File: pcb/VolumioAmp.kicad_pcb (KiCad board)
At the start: 2 copper layers, 172.1 x 71.1 mm, 121 parts, among them IC1 PCM2706, IC2 WM8804GEDS_V, J1 L829-1J1T-43, J2 USB4500-03-0-A_REVA, J3 24v Input, J4 Screw_Terminal_01x04, J5 Conn_Coaxial, Q1 DMP3013SFV-7, U1 74LVC1G07SE-7, U2 TPD4EUSB30, U3 TPD4EUSB30, U4 FSUSB42MUX, U5 24AA02-OT, U6 AP64501SP-13, U7 LT1761-3.3, U8 MA12040PXUMA1, Y1 12Mhz, Y2 12Mhz

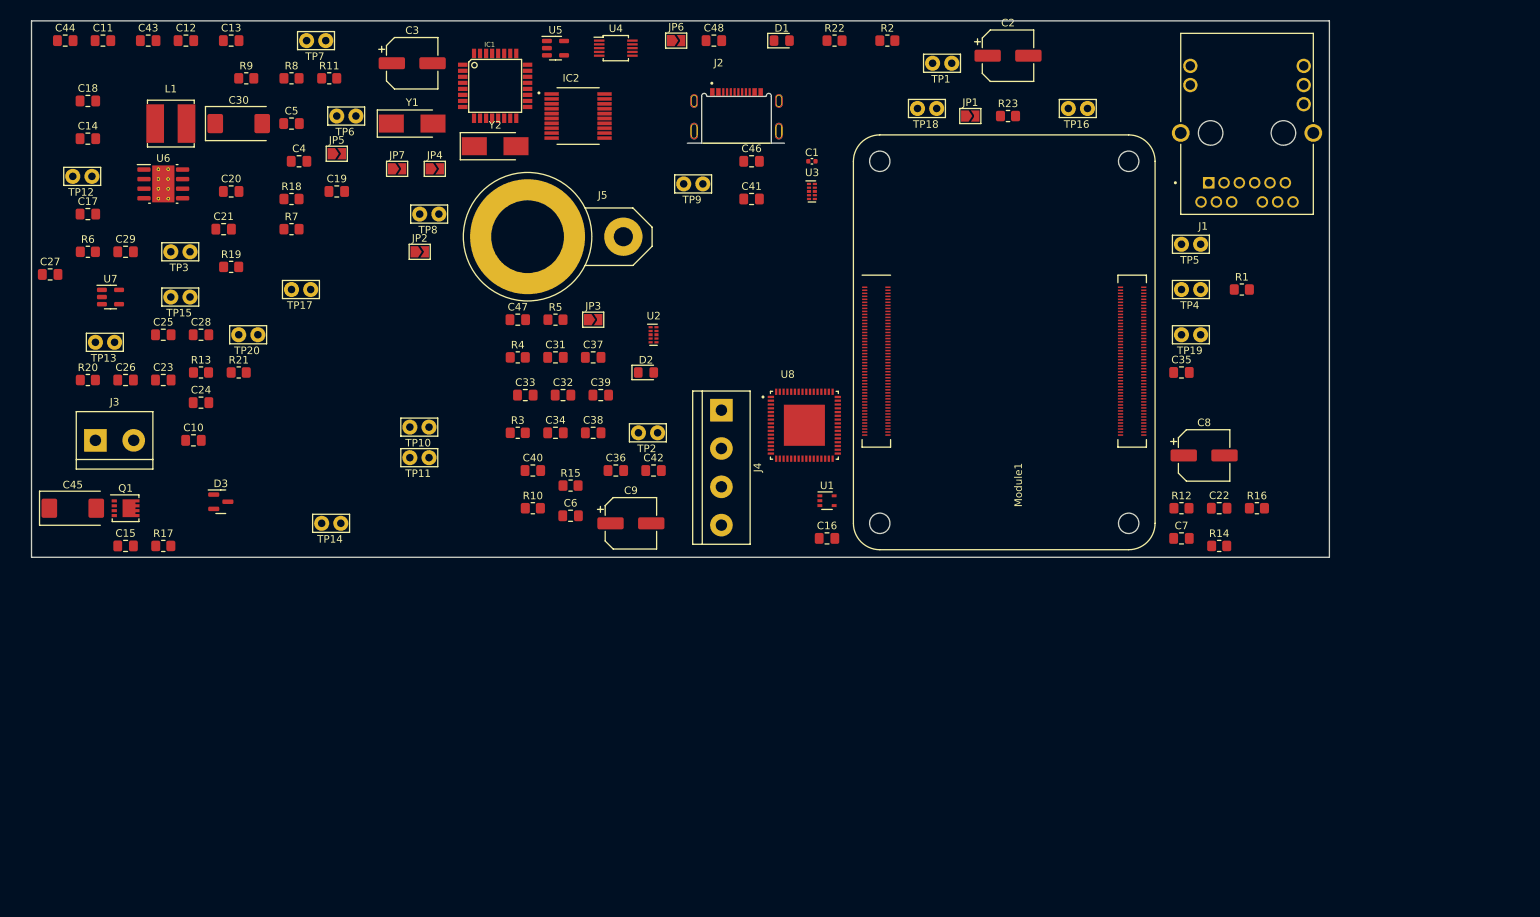
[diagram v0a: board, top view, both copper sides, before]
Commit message: - placing components
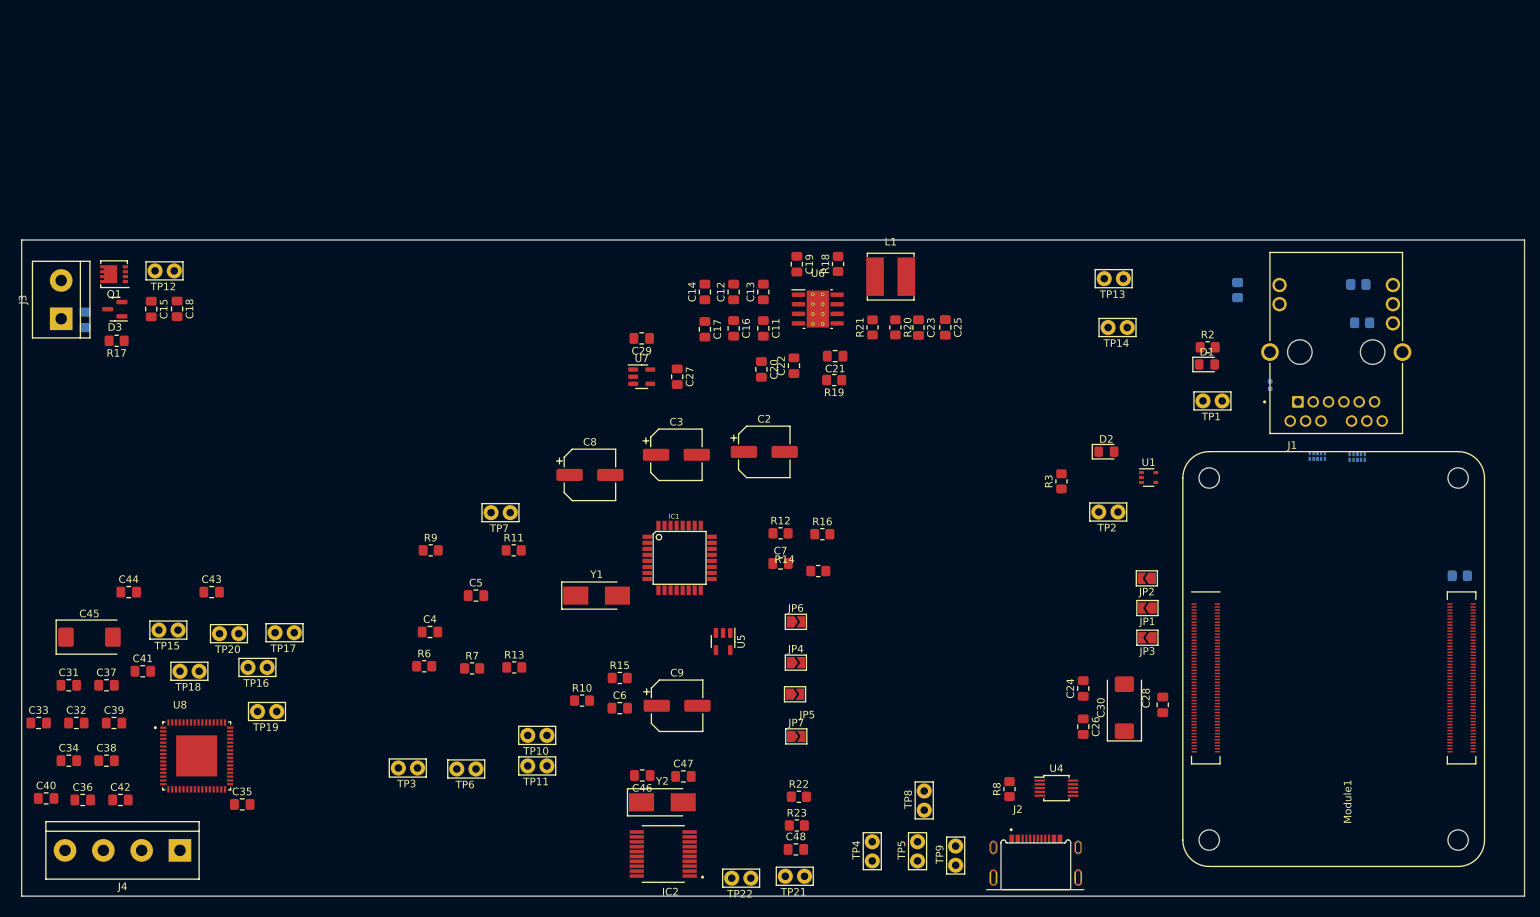
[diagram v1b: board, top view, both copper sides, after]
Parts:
- removed J5: Conn_Coaxial, Connector_Coaxial:BNC_PanelMountable_Vertical
- added R24: 470R, Resistor_SMD:R_0805_2012Metric_Pad1.20x1.40mm_HandSolder, B.Cu at (209.5, 59.3)
- added TP21: TestPoint, TestPoint:TestPoint_Bridge_Pitch2.54mm_Drill1.0mm, F.Cu at (133.5, 137.8)
- added TP22: TestPoint, TestPoint:TestPoint_Bridge_Pitch2.54mm_Drill1.0mm, F.Cu at (126.4, 138.0)
- C1, C10, R1, R4, R5, U2, U3: moved to B.Cu
- R8: value 2.2K 1% -> 2.2K
- moved C30 140.7 mm to (178.4, 115.4), turned to 90 degrees
- moved C35 137.1 mm to (61.5, 128.3)
- moved C28 136.6 mm to (183.5, 115.1), turned to 90 degrees
- moved C26 135.0 mm to (173.0, 118.0), turned to -90 degrees
- moved TP13 134.0 mm to (175.8, 58.6)
- moved R8 134.0 mm to (163.2, 126.2), turned to 90 degrees
- moved TP19 132.3 mm to (63.5, 116.0)
- moved TP16 131.6 mm to (62.2, 110.1)
- moved TP18 123.0 mm to (53.2, 110.6)
- moved C24 123.0 mm to (173.0, 112.9), turned to 90 degrees
- moved U4 114.2 mm to (169.4, 126.1)
- moved R4 112.1 mm to (210.0, 64.4), turned to 180 degrees
- moved C48 107.8 mm to (134.9, 134.2)
- moved TP14 107.5 mm to (176.3, 65.0)
- moved R20 107.3 mm to (148.1, 65.0), turned to -90 degrees
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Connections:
- J1 pad 17: unconnected-(J1-Pad17) -> Net-(J1-Pad17)
- Module1 pad 19: unconnected-(Module1A-Ethernet_nLED1(3.3v)-Pad19) -> Net-(Module1A-Ethernet_nLED1(3.3v))
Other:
- board size 172.1 x 71.1 mm -> 199.3 x 87 mm
